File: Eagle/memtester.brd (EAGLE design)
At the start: 80.1 x 23.2 mm, 4 parts

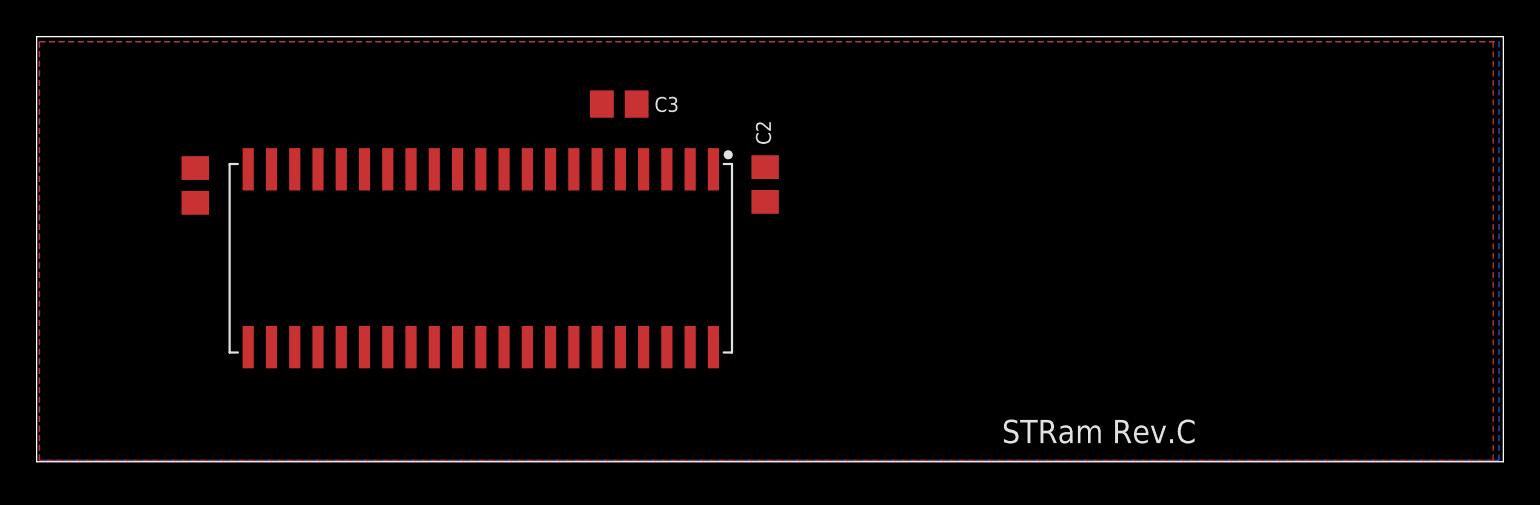
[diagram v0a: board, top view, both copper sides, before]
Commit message: Memtester: part work backup
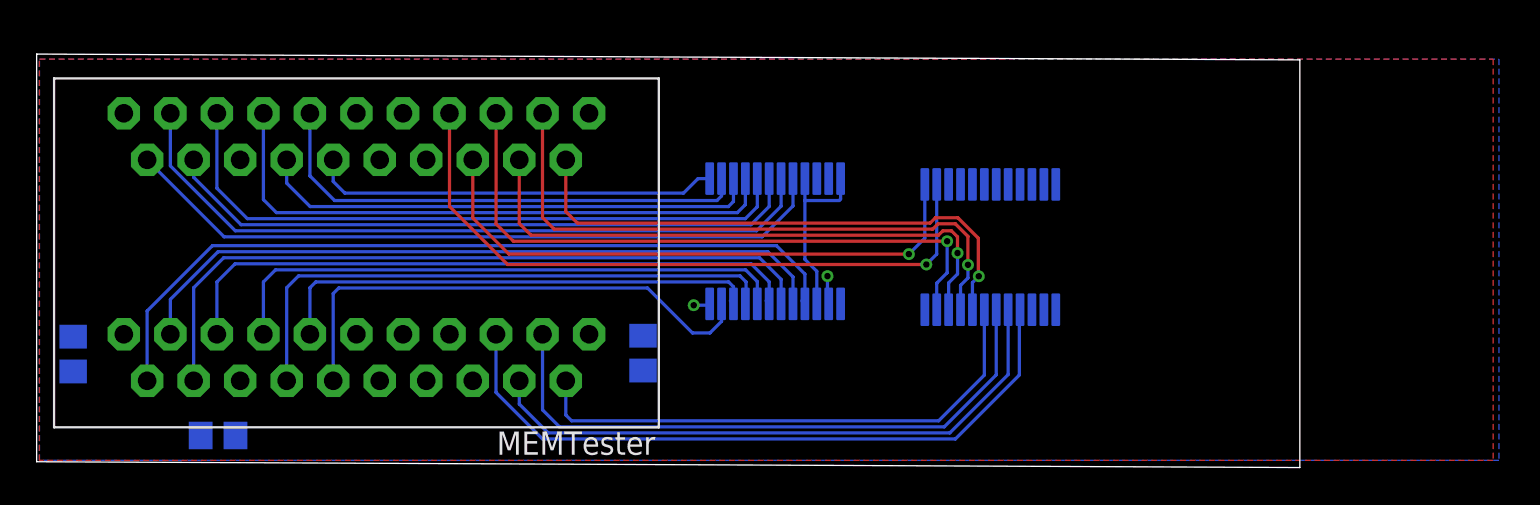
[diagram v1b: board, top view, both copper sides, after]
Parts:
- added U$2, U$3: PCF8575TS, PCF8575TS:SSOP24
- U$1: value NN5118160AJ -> NN5118160AJSOCKET; device AtariST:SOJ127P1117X376-42 -> memory:SOJ42SOCKET
- moved C3 28.4 mm to (9.91, 1.46), flipped to the bottom
- moved C2 11.4 mm to (33.1, 5.96), flipped to the bottom
- moved C1 11.4 mm to (1.99, 5.90), flipped to the bottom
- moved U$1 6.85 mm to (17.5, 12.1), turned to 0 degrees
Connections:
- new net A0: U$1.17, U$3.4
- new net A1: U$1.18, U$3.5
- new net A2: U$1.19, U$3.6
- new net A3: U$1.20, U$3.7
- new net A4: U$1.23, U$3.8
- new net A5: U$1.24, U$3.9
- new net A6: U$1.25, U$3.10
- new net A7: U$1.26, U$3.11
- new net A8: U$1.27, U$3.13
- new net A9: U$1.28, U$3.14
- new net D0: U$1.2, U$2.4
- new net D1: U$1.3, U$2.5
- new net D10: U$1.35, U$2.15
- new net D11: U$1.36, U$2.16
- new net D12: U$1.38, U$2.17
- new net D13: U$1.39, U$2.18
- new net D14: U$1.40, U$2.19
- new net D15: U$1.41, U$2.20
- new net D2: U$1.4, U$2.6
- new net D3: U$1.5, U$2.7
- new net D4: U$1.7, U$2.8
- new net D5: U$1.8, U$2.9
- new net D6: U$1.9, U$2.10
- new net D7: U$1.10, U$2.11
- new net D8: U$1.33, U$2.13
- new net D9: U$1.34, U$2.14
- new net I2C_SCL: U$2.22, U$3.22
- new net I2C_SDA: U$2.23, U$3.23
- net +5V: now also U$2.21, U$2.24, U$2.3, U$3.24, U$3.3
- net GND: now also U$2.12, U$2.2, U$3.12, U$3.2, U$3.21
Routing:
- net D0: track 0.00 -> 43.7 mm
- net D14: track 0.00 -> 39.7 mm
- net D2: track 0.00 -> 39.7 mm
- net D15: track 0.00 -> 39.2 mm
- net D1: track 0.00 -> 39.0 mm
- net A0: track 0.00 -> 37.8 mm
- net A9: track 0.00 -> 37.0 mm, vias 0 -> 1
- net D12: track 0.00 -> 36.1 mm
- net D13: track 0.00 -> 35.4 mm
- net D3: track 0.00 -> 35.3 mm
- net A7: track 0.00 -> 35.0 mm, vias 0 -> 1
- net A2: track 0.00 -> 34.0 mm
- net A5: track 0.00 -> 33.8 mm, vias 0 -> 1
- net A1: track 0.00 -> 33.5 mm
- net D11: track 0.00 -> 32.9 mm
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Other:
- board size 80.1 x 23.2 mm -> 69 x 22.6 mm
- board text added: "MEMTester"
- board text removed: "STRam Rev.C"
